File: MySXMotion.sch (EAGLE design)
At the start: 18 parts, among them IC2 BH1750

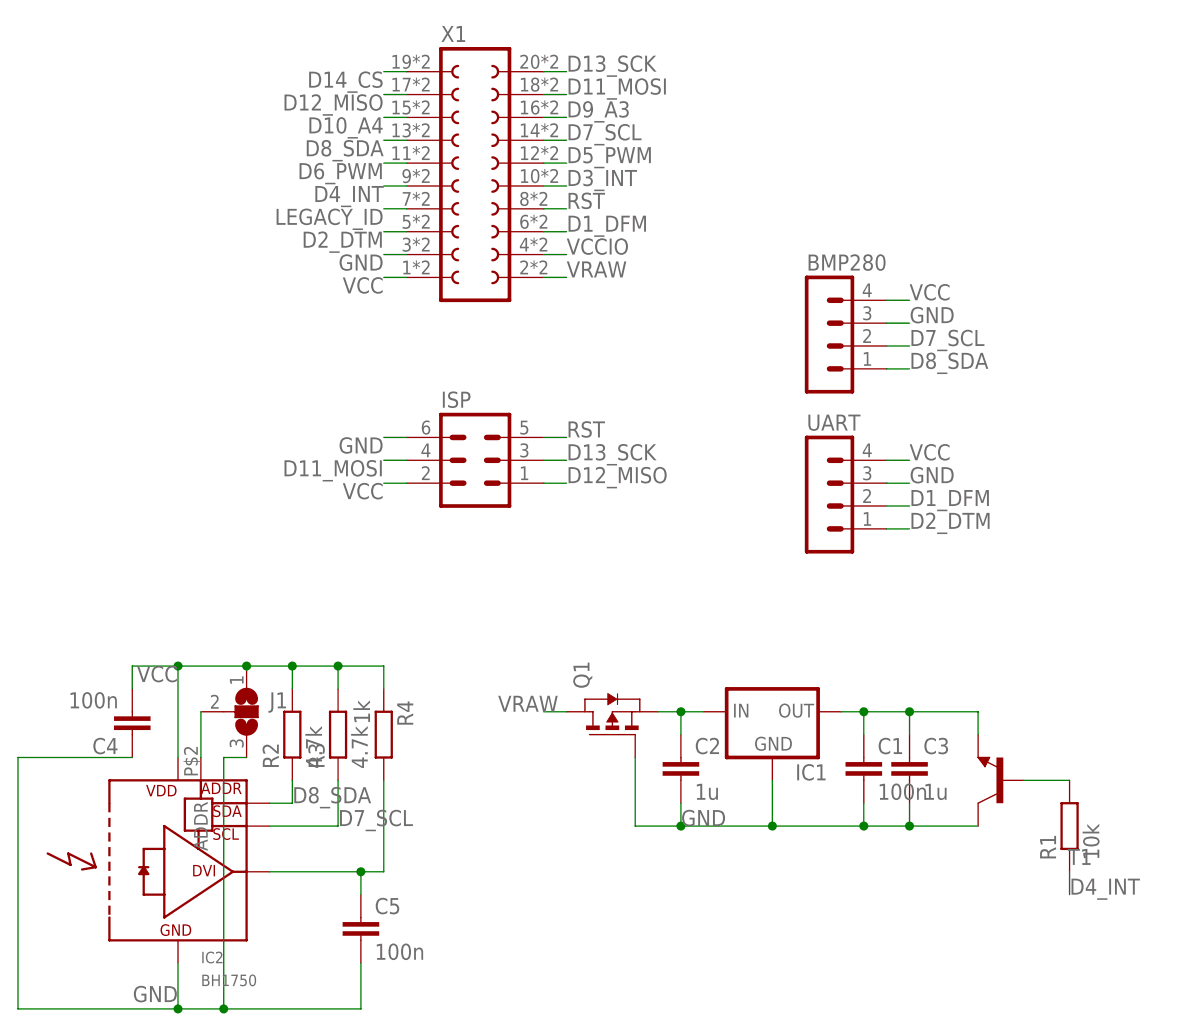
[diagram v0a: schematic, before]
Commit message: add documentation
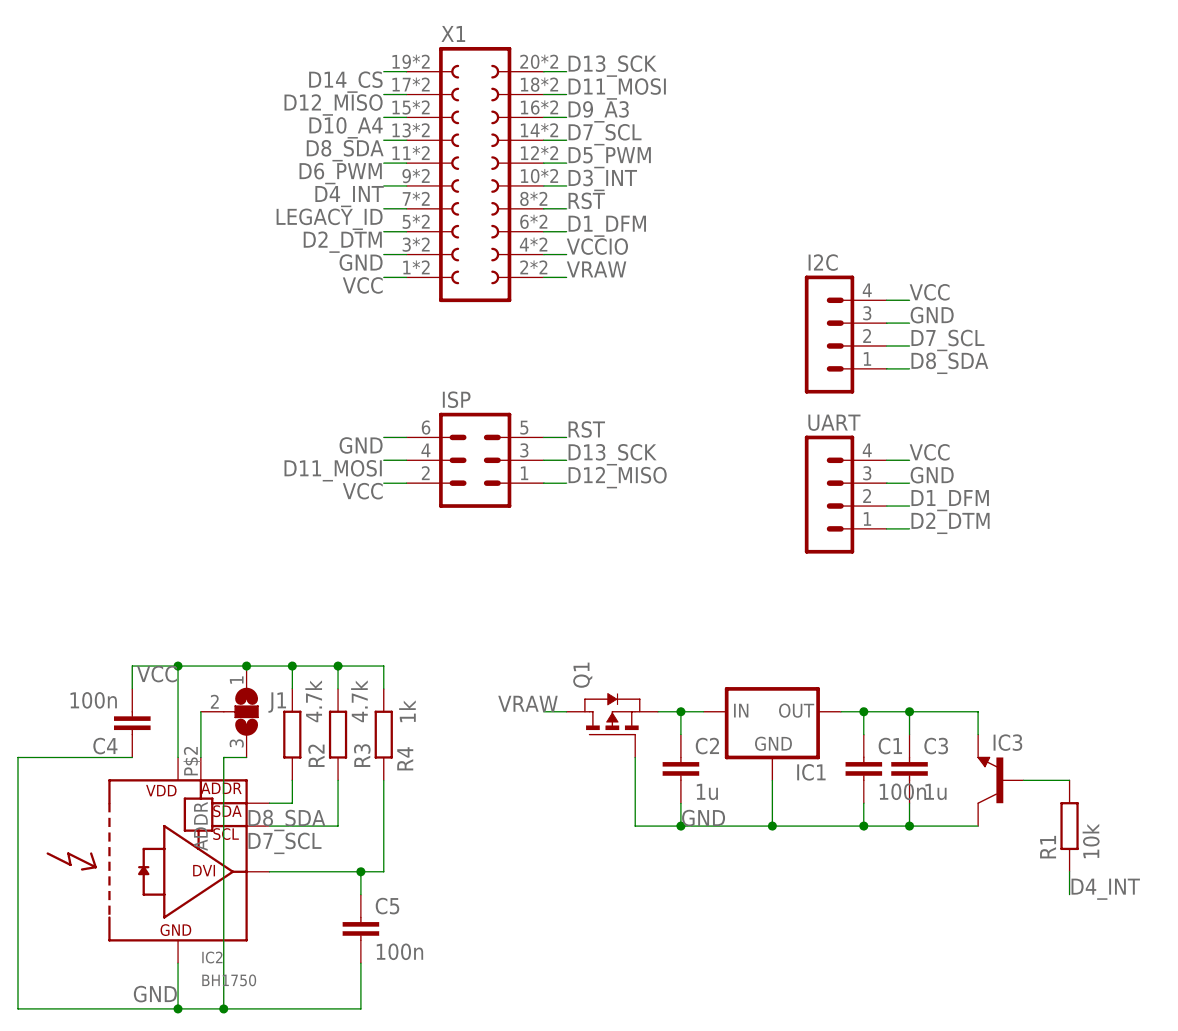
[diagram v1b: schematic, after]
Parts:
- renumbered BMP280 to I2C, T1 to IC3
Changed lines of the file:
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@@
 </classes>
 <parts>
-<part name="BMP280" library="con-lstb" deviceset="MA04-1" device=""/>
+<part name="I2C" library="con-lstb" deviceset="MA04-1" device=""/>
 <part name="ISP" library="con-lstb" deviceset="MA03-2" device=""/>
 <part name="UART" library="con-lstb" deviceset="MA04-1" device=""/>
@@
 <part name="C2" library="rcl" deviceset="C-EU" device="C0603" value="1u"/>
 <part name="C3" library="rcl" deviceset="C-EU" device="C0805" value="1u"/>
-<part name="T1" library="transistor" deviceset="*-NPN-" device="TO5"/>
+<part name="IC3" library="transistor" deviceset="*-NPN-" device="TO5"/>
 <part name="R2" library="rcl" deviceset="R-EU_" device="R0603" value="4.7k"/>
 <part name="R3" library="rcl" deviceset="R-EU_" device="R0603" value="4.7k"/>
@@
 </plain>
 <instances>
-<instance part="BMP280" gate="1" x="48.26" y="43.18"/>
+<instance part="I2C" gate="1" x="48.26" y="43.18"/>
 <instance part="ISP" gate="1" x="10.16" y="27.94"/>
 <instance part="UART" gate="1" x="48.26" y="25.4"/>
@@
 <instance part="C2" gate="G$1" x="33.02" y="-5.08"/>
 <instance part="C3" gate="G$1" x="58.42" y="-5.08"/>
-<instance part="T1" gate="G$1" x="68.58" y="-7.62" rot="R180"/>
-<instance part="R2" gate="G$1" x="-10.16" y="-2.54" rot="R90"/>
-<instance part="R3" gate="G$1" x="-5.08" y="-2.54" rot="R90"/>
+<instance part="IC3" gate="G$1" x="68.58" y="-7.62" smashed="yes" rot="R180">
+<attribute name="NAME" x="71.12" y="-2.54" size="1.778" layer="95" rot="R180"/>
+<attribute name="VALUE" x="78.74" y="-12.7" size="1.778" layer="96" rot="R180"/>
+</instance>
+<instance part="R2" gate="G$1" x="-10.16" y="-2.54" smashed="yes" rot="R90">
+<attribute name="NAME" x="-6.5786" y="-6.35" size="1.778" layer="95" rot="R90"/>
+<attribute name="VALUE" x="-6.858" y="-1.27" size="1.778" layer="96" rot="R90"/>
+</instance>
+<instance part="R3" gate="G$1" x="-5.08" y="-2.54" smashed="yes" rot="R90">
+<attribute name="NAME" x="-1.4986" y="-6.35" size="1.778" layer="95" rot="R90"/>
+<attribute name="VALUE" x="-1.778" y="-1.27" size="1.778" layer="96" rot="R90"/>
+</instance>
 <instance part="C4" gate="G$1" x="-27.94" y="-2.54" rot="R180"/>
-<instance part="R4" gate="G$1" x="0" y="-2.54" rot="R270"/>
+<instance part="R4" gate="G$1" x="0" y="-2.54" smashed="yes" rot="R270">
+<attribute name="NAME" x="1.4986" y="-3.81" size="1.778" layer="95" rot="R270"/>
+<attribute name="VALUE" x="1.778" y="1.27" size="1.778" layer="96" rot="R270"/>
+</instance>
 <instance part="C5" gate="G$1" x="-2.54" y="-22.86"/>
 <instance part="J1" gate="G$1" x="-15.24" y="0"/>
@@
 <net name="VCC" class="1">
 <segment>
-<pinref part="BMP280" gate="1" pin="4"/>
+<pinref part="I2C" gate="1" pin="4"/>
 <wire x1="55.88" y1="45.72" x2="58.42" y2="45.72" width="0.1524" layer="91"/>
 <label x="58.42" y="45.72" size="1.778" layer="95"/>
@@
 <net name="D7_SCL" class="0">
 <segment>
-<pinref part="BMP280" gate="1" pin="2"/>
+<pinref part="I2C" gate="1" pin="2"/>
 <wire x1="55.88" y1="40.64" x2="58.42" y2="40.64" width="0.1524" layer="91"/>
 <label x="58.42" y="40.64" size="1.778" layer="95"/>
@@
 <wire x1="-12.7" y1="-12.7" x2="-5.08" y2="-12.7" width="0.1524" layer="91"/>
 <wire x1="-5.08" y1="-12.7" x2="-5.08" y2="-7.62" width="0.1524" layer="91"/>
-<label x="-5.08" y="-12.7" size="1.778" layer="95"/>
+<label x="-15.24" y="-15.24" size="1.778" layer="95"/>
 </segment>
 </net>
@@
 <net name="D8_SDA" class="0">
 <segment>
-<pinref part="BMP280" gate="1" pin="1"/>
+<pinref part="I2C" gate="1" pin="1"/>
 <wire x1="55.88" y1="38.1" x2="58.42" y2="38.1" width="0.1524" layer="91"/>
 <label x="58.42" y="38.1" size="1.778" layer="95"/>
@@
 <wire x1="-12.7" y1="-10.16" x2="-10.16" y2="-10.16" width="0.1524" layer="91"/>
 <wire x1="-10.16" y1="-10.16" x2="-10.16" y2="-7.62" width="0.1524" layer="91"/>
-<label x="-10.16" y="-10.16" size="1.778" layer="95"/>
+<label x="-15.24" y="-12.7" size="1.778" layer="95"/>
 </segment>
 </net>
@@
 <net name="GND" class="1">
 <segment>
-<pinref part="BMP280" gate="1" pin="3"/>
+<pinref part="I2C" gate="1" pin="3"/>
 <wire x1="55.88" y1="43.18" x2="58.42" y2="43.18" width="0.1524" layer="91"/>
 <label x="58.42" y="43.18" size="1.778" layer="95"/>
@@
 <wire x1="43.18" y1="-7.62" x2="43.18" y2="-12.7" width="0.1524" layer="91"/>
 <label x="33.02" y="-12.7" size="1.778" layer="95"/>
-<pinref part="T1" gate="G$1" pin="C"/>
+<pinref part="IC3" gate="G$1" pin="C"/>
 <wire x1="66.04" y1="-12.7" x2="58.42" y2="-12.7" width="0.1524" layer="91"/>
 <junction x="43.18" y="-12.7"/>
@@
 <wire x1="58.42" y1="0" x2="58.42" y2="-2.54" width="0.1524" layer="91"/>
 <wire x1="58.42" y1="0" x2="66.04" y2="0" width="0.1524" layer="91"/>
-<pinref part="T1" gate="G$1" pin="E"/>
+<pinref part="IC3" gate="G$1" pin="E"/>
 <wire x1="66.04" y1="-2.54" x2="66.04" y2="0" width="0.1524" layer="91"/>
 <junction x="53.34" y="0"/>
@@
 <segment>
 <pinref part="R1" gate="G$1" pin="2"/>
-<pinref part="T1" gate="G$1" pin="B"/>
+<pinref part="IC3" gate="G$1" pin="B"/>
 <wire x1="76.2" y1="-7.62" x2="71.12" y2="-7.62" width="0.1524" layer="91"/>
 </segment>
